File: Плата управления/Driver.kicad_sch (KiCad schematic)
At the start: 24 parts, among them U1 IR2184, U2 IR2184, U3 IR2184

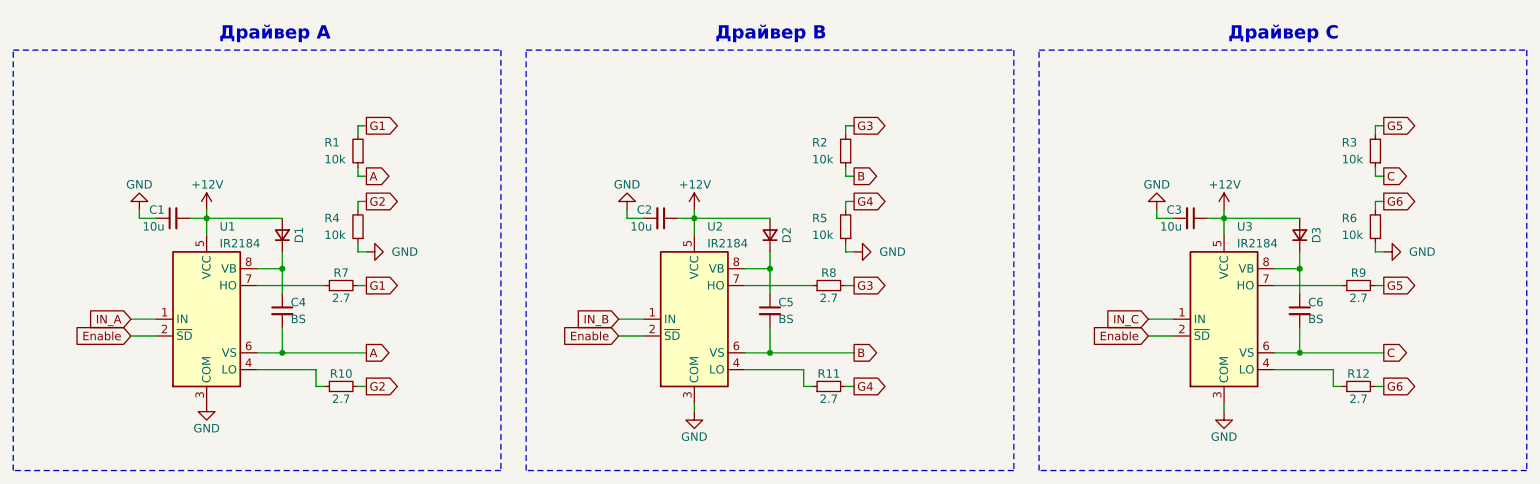
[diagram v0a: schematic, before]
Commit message: Версия под отчёт
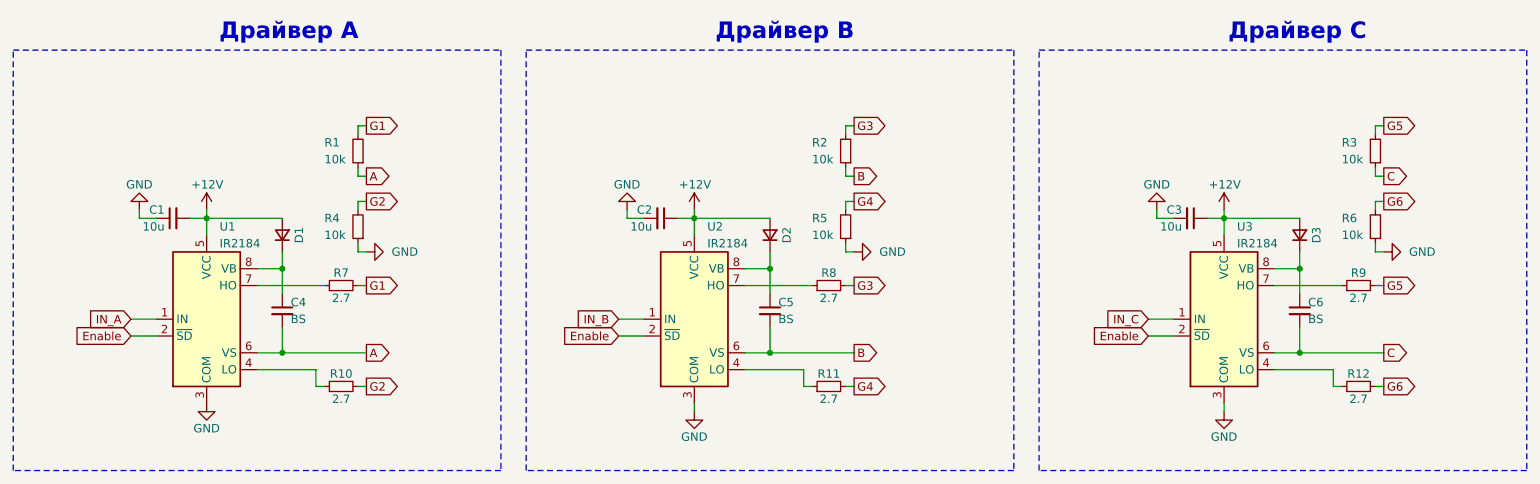
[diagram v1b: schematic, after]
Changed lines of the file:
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@@
   )
   (text "Драйвер С" (at 221.615 66.04 0)
-    (effects (font (size 2 2) (thickness 0.254) bold) (justify left bottom))
+    (effects (font (size 2.5 2.5) (thickness 0.254) bold) (justify left bottom))
   )
   (text "Драйвер А" (at 69.215 66.04 0)
-    (effects (font (size 2 2) (thickness 0.254) bold) (justify left bottom))
+    (effects (font (size 2.5 2.5) (thickness 0.254) bold) (justify left bottom))
   )
   (text "Драйвер В" (at 144.145 66.04 0)
-    (effects (font (size 2 2) (thickness 0.254) bold) (justify left bottom))
+    (effects (font (size 2.5 2.5) (thickness 0.254) bold) (justify left bottom))
   )
   (global_label "IN_A" (shape input) (at 55.88 107.95 180) (fields_autoplaced)
